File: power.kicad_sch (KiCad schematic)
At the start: 13 parts, among them J2 USB_C_Receptacle_PowerOnly_6P

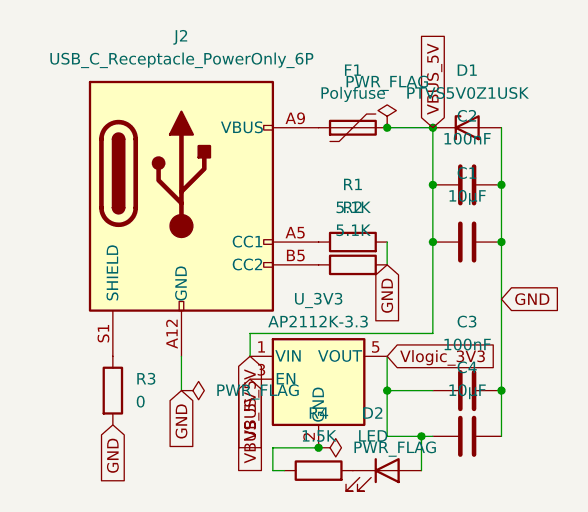
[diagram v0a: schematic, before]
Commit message: Add files via upload
v1.2 : complete schematics with added footprints, PCB layout remaining
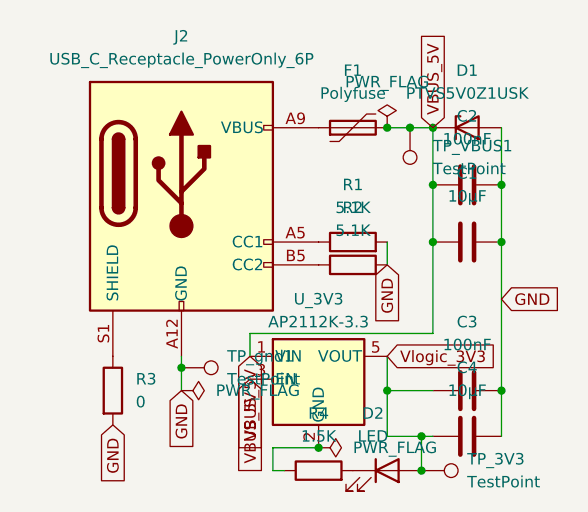
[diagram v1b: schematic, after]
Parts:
- added TP_3V3, TP_VBUS1, TP_gnd1: TestPoint, TestPoint:TestPoint_Pad_D1.5mm, symbol Connector:TestPoint
- F1: footprint (none) -> Fuse:Fuse_1206_3216Metric
- J2: footprint (none) -> Connector_USB:USB_C_Receptacle_HRO_TYPE-C-31-M-12
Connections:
- net GND: now also TP_gnd1.1
- net VBUS_5V: now also TP_VBUS1.1
- net Vlogic_3V3: now also TP_3V3.1
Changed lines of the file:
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@@
+	)
+	(junction
+		(at 147.32 69.85)
+		(diameter 0)
+		(color 0 0 0 0)
 	)
 	(junction
@@
 	)
 	(junction
+		(at 120.65 58.42)
+		(diameter 0)
+		(color 0 0 0 0)
+	)
+	(junction
 		(at 156.21 60.96)
 		(diameter 0)
@@
 	)
 	(junction
+		(at 146.05 31.75)
+		(diameter 0)
+		(color 0 0 0 0)
+	)
+	(junction
 		(at 156.21 44.45)
 		(diameter 0)
@@
 	(wire
 		(pts
+			(xy 120.65 58.42) (xy 120.65 57.15)
+		)
+		(stroke
+			(width 0)
+			(type default)
+		)
+	)
+	(wire
+		(pts
 			(xy 156.21 38.1) (xy 156.21 44.45)
 		)
@@
 	(wire
 		(pts
+			(xy 146.05 31.75) (xy 148.59 31.75)
+		)
+		(stroke
+			(width 0)
+			(type default)
+		)
+	)
+	(wire
+		(pts
 			(xy 147.32 66.04) (xy 147.32 69.85)
 		)
@@
 	(wire
 		(pts
-			(xy 143.51 31.75) (xy 148.59 31.75)
+			(xy 143.51 31.75) (xy 146.05 31.75)
 		)
 		(stroke
@@
 	(wire
 		(pts
-			(xy 120.65 60.96) (xy 120.65 57.15)
+			(xy 120.65 60.96) (xy 120.65 58.42)
 		)
 		(stroke
@@
 	)
 	(symbol
+		(lib_id "Connector:TestPoint")
+		(at 146.05 31.75 180)
+		(unit 1)
+		(exclude_from_sim no)
+		(in_bom yes)
+		(on_board yes)
+		(dnp no)
+		(fields_autoplaced yes)
+		(property "Reference" "TP_VBUS1"
+			(at 148.59 33.7819 0)
+			(effects
+				(font
+					(size 1.27 1.27)
+				)
+				(justify right)
+			)
+		)
+		(property "Value" "TestPoint"
+			(at 148.59 36.3219 0)
+			(effects
+				(font
+					(size 1.27 1.27)
+				)
+				(justify right)
+			)
+		)
+		(property "Footprint" "TestPoint:TestPoint_Pad_D1.5mm"
+			(at 140.97 31.75 0)
+			(effects
+				(font
+					(size 1.27 1.27)
+				)
+				(hide yes)
+			)
+		)
+		(property "Datasheet" "~"
+			(at 140.97 31.75 0)
+			(effects
+				(font
+					(size 1.27 1.27)
+				)
+				(hide yes)
+			)
+		)
+		(property "Description" "test point"
+			(at 146.05 31.75 0)
+			(effects
+				(font
+					(size 1.27 1.27)
+				)
+				(hide yes)
+			)
+		)
+		(pin "1"
+		)
+		(instances
+			(project ""
+				(path "/c8d0e3cf-b697-430c-b4f3-c5285558b4ca/a3d1f251-0cce-4493-9b12-767abad6ca7c"
+					(reference "TP_VBUS1")
+					(unit 1)
+				)
+			)
+		)
+	)
+	(symbol
 		(lib_id "Device:R")
 		(at 113.03 60.96 0)
@@
 			)
 		)
-		(property "Footprint" ""
+		(property "Footprint" "Connector_USB:USB_C_Receptacle_HRO_TYPE-C-31-M-12"
 			(at 124.46 36.83 0)
 			(effects
@@
 			)
 		)
-		(property "Footprint" ""
+		(property "Footprint" "Fuse:Fuse_1206_3216Metric"
 			(at 144.78 30.48 0)
 			(effects
@@
 					(unit 1)
 				)
+			)
+		)
+	)
+	(symbol
+		(lib_id "Connector:TestPoint")
+		(at 147.32 69.85 270)
+		(unit 1)
+		(exclude_from_sim no)
+		(in_bom yes)
+		(on_board yes)
+		(dnp no)
+		(fields_autoplaced yes)
+		(property "Reference" "TP_3V3"
+			(at 152.4 68.5799 90)
+			(effects
+				(font
+					(size 1.27 1.27)
+				)
+				(justify left)
+			)
+		)
+		(property "Value" "TestPoint"
+			(at 152.4 71.1199 90)
+			(effects
+				(font
+					(size 1.27 1.27)
+				)
+				(justify left)
+			)
+		)
+		(property "Footprint" "TestPoint:TestPoint_Pad_D1.5mm"
+			(at 147.32 74.93 0)
+			(effects
+				(font
+					(size 1.27 1.27)
+				)
+				(hide yes)
+			)
+		)
+		(property "Datasheet" "~"
+			(at 147.32 74.93 0)
+			(effects
+				(font
+					(size 1.27 1.27)
+				)
+				(hide yes)
+			)
+		)
+		(property "Description" "test point"
+			(at 147.32 69.85 0)
+			(effects
+				(font
+					(size 1.27 1.27)
+				)
+				(hide yes)
+			)
+		)
+		(pin "1"
+		)
+		(instances
+			(project ""
+				(path "/c8d0e3cf-b697-430c-b4f3-c5285558b4ca/a3d1f251-0cce-4493-9b12-767abad6ca7c"
+					(reference "TP_3V3")
+					(unit 1)
+				)
+			)
+		)
+	)
+	(symbol
+		(lib_id "Connector:TestPoint")
+		(at 120.65 58.42 270)
+		(unit 1)
+		(exclude_from_sim no)
+		(in_bom yes)
+		(on_board yes)
+		(dnp no)
+		(fields_autoplaced yes)
+		(property "Reference" "TP_gnd1"
+			(at 125.73 57.1499 90)
+			(effects
+				(font
+					(size 1.27 1.27)
+				)
+				(justify left)
+			)
+		)
+		(property "Value" "TestPoint"
+			(at 125.73 59.6899 90)
+			(effects
+				(font
+					(size 1.27 1.27)
+				)
+				(justify left)
+			)
+		)
+		(property "Footprint" "TestPoint:TestPoint_Pad_D1.5mm"
+			(at 120.65 63.5 0)
+			(effects
+				(font
+					(size 1.27 1.27)
+				)
+				(hide yes)
+			)
+		)
+		(property "Datasheet" "~"
+			(at 120.65 63.5 0)
+			(effects
+				(font
+					(size 1.27 1.27)
+				)
+				(hide yes)
+			)
+		)
+		(property "Description" "test point"
+			(at 120.65 58.42 0)
+			(effects
+				(font
+					(size 1.27 1.27)
+				)
+				(hide yes)
+			)
+		)
+		(pin "1"
+		)
+		(instances
+			(project ""
+				(path "/c8d0e3cf-b697-430c-b4f3-c5285558b4ca/a3d1f251-0cce-4493-9b12-767abad6ca7c"
+					(reference "TP_gnd1")
+					(unit 1)
+				)
